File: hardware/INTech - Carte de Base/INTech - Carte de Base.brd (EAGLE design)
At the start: 160 x 107.6 mm, 41 parts

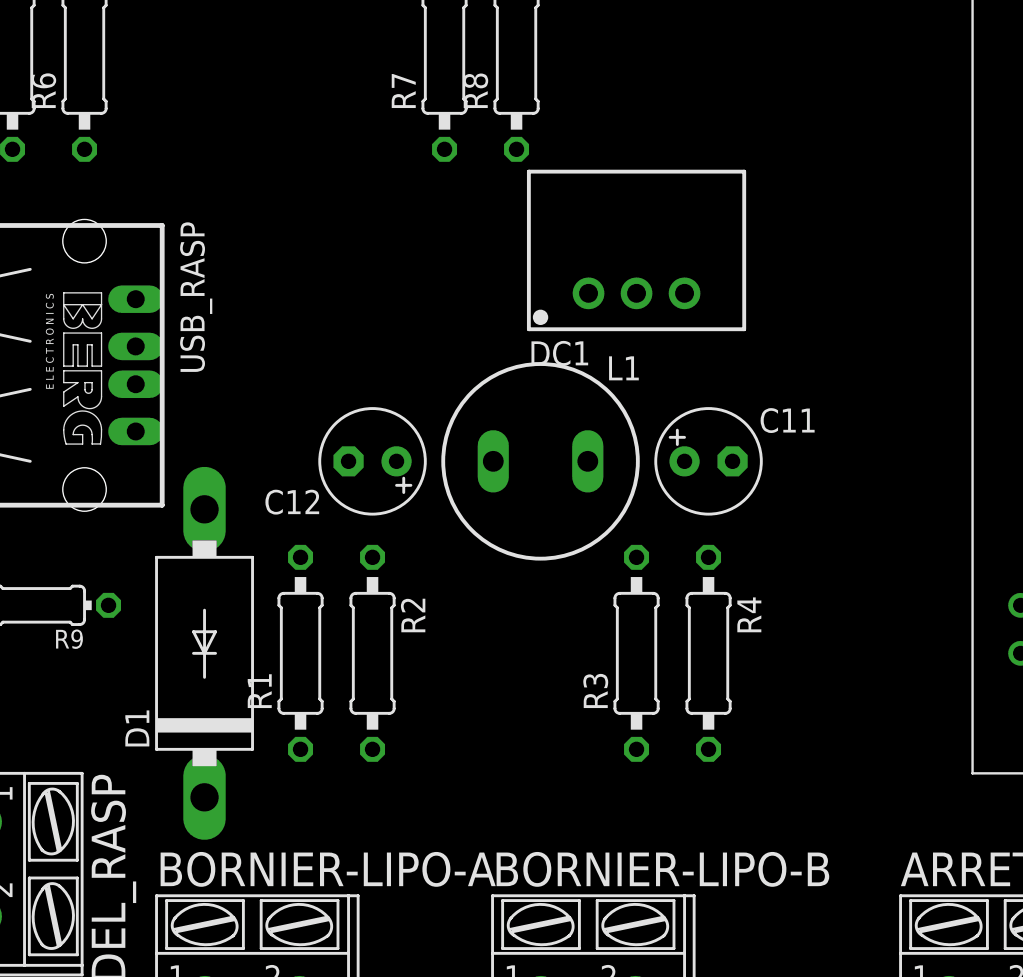
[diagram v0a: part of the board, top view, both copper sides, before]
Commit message: Ajout de texte pour les régulateurs de tension
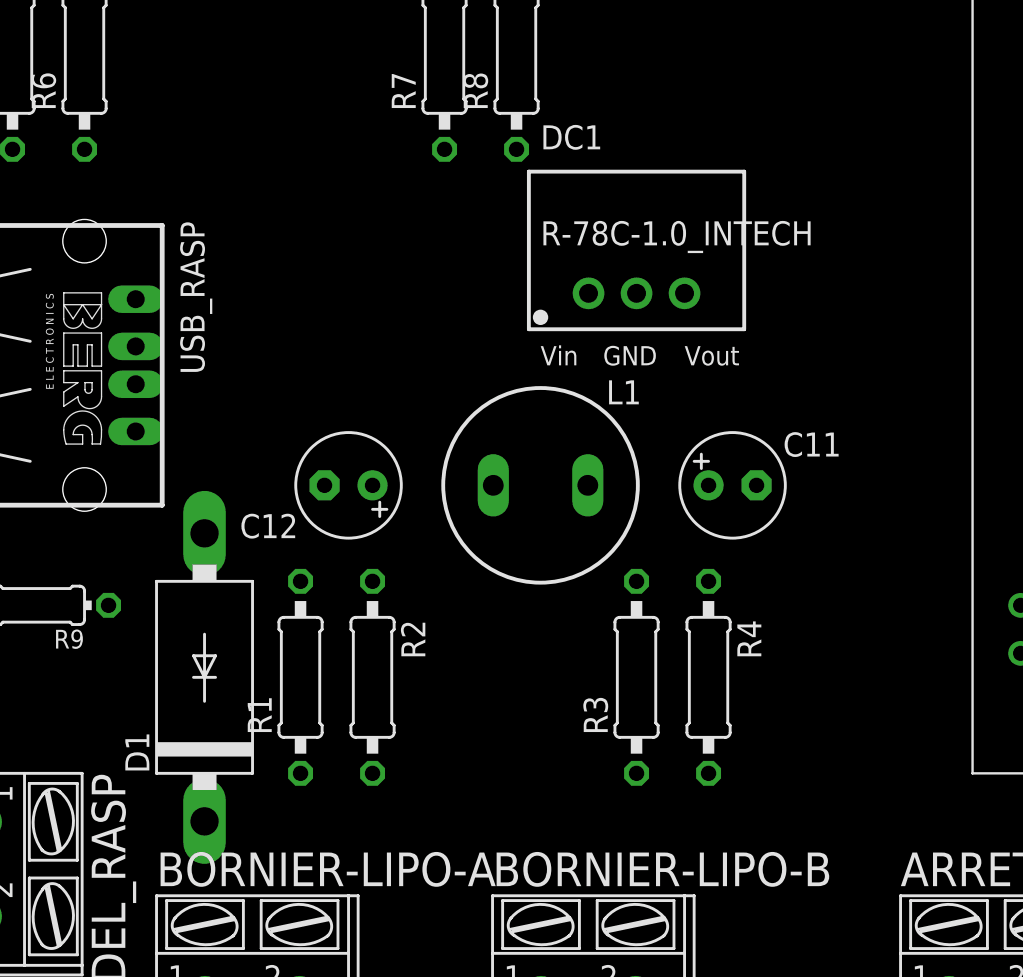
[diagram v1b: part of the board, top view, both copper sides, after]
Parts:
- DC1: value R-78C5.0-1.0 -> R-78C-1.0_INTECH; device dc-dc-converter:SIP3 -> dc-dc-converter:SIP3_INTECH
- moved C12 1.80 mm to (27.9, 36.8)
- moved C11 1.80 mm to (48.3, 36.8)
- moved L1 1.27 mm to (38.1, 36.8)
- moved D1 1.27 mm to (20.3, 26.7)
- moved R1 1.27 mm to (25.4, 26.7)
- moved R2 1.27 mm to (29.2, 26.7)
- moved R3 1.27 mm to (43.2, 26.7)
- moved R4 1.27 mm to (47.0, 26.7)
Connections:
- net +5V_RASP: now also DC1.VOUT; no longer DC1.3
- net GND: now also DC1.GND; no longer DC1.2
- net N$12: now also DC1.VIN; no longer DC1.1
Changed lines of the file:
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@@
 <attribute name="OC_FARNELL" value="unknown" x="22.86" y="8.89" size="1.778" layer="27" display="off"/>
 </element>
-<element name="D1" library="diode" package="DO27-15" value="BYT03" x="20.32" y="27.94" rot="R90"/>
+<element name="D1" library="diode" package="DO27-15" value="BYT03" x="20.32" y="26.67" rot="R90"/>
 <element name="ARRET-LIPOS" library="con-ptr500" package="AK300/2" value="" x="62.23" y="8.89">
 <attribute name="OC_NEWARK" value="unknown" x="62.23" y="8.89" size="1.778" layer="27" display="off"/>
@@
 <attribute name="OC_FARNELL" value="unknown" x="40.64" y="8.89" size="1.778" layer="27" display="off"/>
 </element>
-<element name="R1" library="resistor" package="0207/10" value="" x="25.4" y="27.94" rot="R90"/>
-<element name="R2" library="resistor" package="0207/10" value="" x="29.21" y="27.94" rot="R270"/>
-<element name="R3" library="resistor" package="0207/10" value="27K" x="43.18" y="27.94" rot="R90"/>
-<element name="R4" library="resistor" package="0207/10" value="3.3K" x="46.99" y="27.94" rot="R270"/>
+<element name="R1" library="resistor" package="0207/10" value="" x="25.4" y="26.67" rot="R90"/>
+<element name="R2" library="resistor" package="0207/10" value="" x="29.21" y="26.67" rot="R270"/>
+<element name="R3" library="resistor" package="0207/10" value="27K" x="43.18" y="26.67" rot="R90"/>
+<element name="R4" library="resistor" package="0207/10" value="3.3K" x="46.99" y="26.67" rot="R270"/>
 <element name="SERIE" library="pinhead_CF_INTech" package="PINHEAD_CF_INTECH" value="PINHEAD_CF_INTECH" x="97.79" y="8.89" rot="R180"/>
 <element name="MOTEUR_GAUCHE" library="LM18200T_CF_INTech" package="LM18200T_CF_INTECH" value="LM18200T_CF_INTECH" x="17.78" y="88.9"/>
@@
 <element name="JUMPER" library="pinhead_CF_INTech" package="PINHEAD_CF_INTECH" value="PINHEAD_CF_INTECH" x="109.22" y="12.7"/>
 <element name="R9" library="resistor" package="0204/7" value="470" x="11.43" y="30.48" rot="R180"/>
-<element name="C11" library="resistor" package="E2,5-6" value="10µF" x="46.99" y="38.1"/>
-<element name="C12" library="resistor" package="E2,5-6" value="22µF" x="29.21" y="38.1" rot="R180"/>
-<element name="L1" library="inductor-neosid" package="SD12K100" value="68µH" x="38.1" y="38.1">
-<attribute name="OC_NEWARK" value="unknown" x="38.1" y="38.1" size="1.778" layer="27" display="off"/>
-<attribute name="MPN" value="" x="38.1" y="38.1" size="1.778" layer="27" display="off"/>
-<attribute name="MF" value="" x="38.1" y="38.1" size="1.778" layer="27" display="off"/>
-<attribute name="OC_FARNELL" value="unknown" x="38.1" y="38.1" size="1.778" layer="27" display="off"/>
-</element>
-<element name="DC1" library="dc-dc-converter" package="SIP3" value="R-78C5.0-1.0" x="43.18" y="46.99"/>
+<element name="C11" library="resistor" package="E2,5-6" value="10µF" x="48.26" y="36.83"/>
+<element name="C12" library="resistor" package="E2,5-6" value="22µF" x="27.94" y="36.83" rot="R180"/>
+<element name="L1" library="inductor-neosid" package="SD12K100" value="68µH" x="38.1" y="36.83">
+<attribute name="OC_NEWARK" value="unknown" x="38.1" y="36.83" size="1.778" layer="27" display="off"/>
+<attribute name="MPN" value="" x="38.1" y="36.83" size="1.778" layer="27" display="off"/>
+<attribute name="MF" value="" x="38.1" y="36.83" size="1.778" layer="27" display="off"/>
+<attribute name="OC_FARNELL" value="unknown" x="38.1" y="36.83" size="1.778" layer="27" display="off"/>
+</element>
+<element name="DC1" library="dc-dc-converter" package="SIP3_INTECH" value="R-78C-1.0_INTECH" x="43.18" y="46.99"/>
 <element name="DEL_RASP" library="con-ptr500" package="AK300/2" value="" x="7.62" y="16.51" rot="R270">
 <attribute name="OC_NEWARK" value="unknown" x="7.62" y="16.51" size="1.778" layer="27" rot="R270" display="off"/>
@@
 <contactref element="C12" pad="-"/>
 <contactref element="C11" pad="-"/>
-<contactref element="DC1" pad="2"/>
+<contactref element="DC1" pad="GND"/>
 <contactref element="DEL_RASP" pad="1"/>
 <contactref element="USB_RASP" pad="4"/>
@@
 <contactref element="BORNIER-LIPO-A" pad="1"/>
 <contactref element="D1" pad="C"/>
-<wire x1="20.3454" y1="8.89" x2="20.32" y2="20.32" width="0" layer="19" extent="1-1"/>
+<wire x1="20.3454" y1="8.89" x2="20.32" y2="19.05" width="0" layer="19" extent="1-1"/>
 </signal>
 <signal name="+24V_RASP">
@@
 <contactref element="C12" pad="+"/>
 <contactref element="L1" pad="1"/>
-<wire x1="35.6" y1="38.1" x2="78.7654" y2="8.89" width="0" layer="19" extent="1-1"/>
-<wire x1="30.48" y1="38.1" x2="35.6" y2="38.1" width="0" layer="19" extent="1-1"/>
+<wire x1="35.6" y1="36.83" x2="78.7654" y2="8.89" width="0" layer="19" extent="1-1"/>
+<wire x1="29.21" y1="36.83" x2="35.6" y2="36.83" width="0" layer="19" extent="1-1"/>
 </signal>
 <signal name="+24V">
@@
 <wire x1="59.7154" y1="8.89" x2="83.7692" y2="8.89" width="0" layer="19" extent="1-1"/>
 <wire x1="43.1292" y1="8.89" x2="59.7154" y2="8.89" width="0" layer="19" extent="1-1"/>
-<wire x1="43.18" y1="22.86" x2="43.1292" y2="8.89" width="0" layer="19" extent="1-1"/>
+<wire x1="43.18" y1="21.59" x2="43.1292" y2="8.89" width="0" layer="19" extent="1-1"/>
 </signal>
 <signal name="TEST_LIPO_12V">
 <contactref element="R1" pad="2"/>
 <contactref element="R2" pad="1"/>
-<wire x1="25.4" y1="33.02" x2="29.21" y2="33.02" width="0" layer="19" extent="1-1"/>
+<wire x1="25.4" y1="31.75" x2="29.21" y2="31.75" width="0" layer="19" extent="1-1"/>
 </signal>
 <signal name="+12V_LIPO">
@@
 <contactref element="BORNIER-LIPO-B" pad="1"/>
 <contactref element="R1" pad="1"/>
-<wire x1="25.3492" y1="8.89" x2="25.4" y2="22.86" width="0" layer="19" extent="1-1"/>
-<wire x1="38.1254" y1="8.89" x2="25.3492" y2="8.89" width="0" layer="19" extent="1-1"/>
+<wire x1="25.3492" y1="8.89" x2="38.1254" y2="8.89" width="0" layer="19" extent="1-1"/>
+<wire x1="25.4" y1="21.59" x2="25.3492" y2="8.89" width="0" layer="19" extent="1-1"/>
 </signal>
 <signal name="TEST_LIPO_24V">
 <contactref element="R4" pad="1"/>
 <contactref element="R3" pad="2"/>
-<wire x1="43.18" y1="33.02" x2="46.99" y2="33.02" width="0" layer="19" extent="1-1"/>
+<wire x1="43.18" y1="31.75" x2="46.99" y2="31.75" width="0" layer="19" extent="1-1"/>
 </signal>
 <signal name="UART_ROUGE">
@@
 </signal>
 <signal name="N$12">
-<contactref element="DC1" pad="1"/>
+<contactref element="DC1" pad="VIN"/>
 <contactref element="C11" pad="+"/>
 <contactref element="L1" pad="2"/>
-<wire x1="40.6" y1="38.1" x2="40.64" y2="46.99" width="0" layer="19" extent="1-1"/>
-<wire x1="45.72" y1="38.1" x2="40.6" y2="38.1" width="0" layer="19" extent="1-1"/>
+<wire x1="40.6" y1="36.83" x2="40.64" y2="46.99" width="0" layer="19" extent="1-1"/>
+<wire x1="46.99" y1="36.83" x2="40.6" y2="36.83" width="0" layer="19" extent="1-1"/>
 </signal>
 <signal name="N$16">
@@
 <signal name="+5V_RASP">
 <contactref element="USB_RASP" pad="1"/>
-<contactref element="DC1" pad="3"/>
+<contactref element="DC1" pad="VOUT"/>
 <contactref element="R9" pad="1"/>
 <wire x1="16.68" y1="46.68" x2="45.72" y2="46.99" width="0" layer="19" extent="1-1"/>
